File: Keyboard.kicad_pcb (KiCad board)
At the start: 2 copper layers, 50.8 x 59.5 mm, 36 parts, among them SW1 SW_Push, SW2 SW_Push, SW3 SW_Push, U1 ATmega32U2-AU, Y1 Crystal_GND24_Small

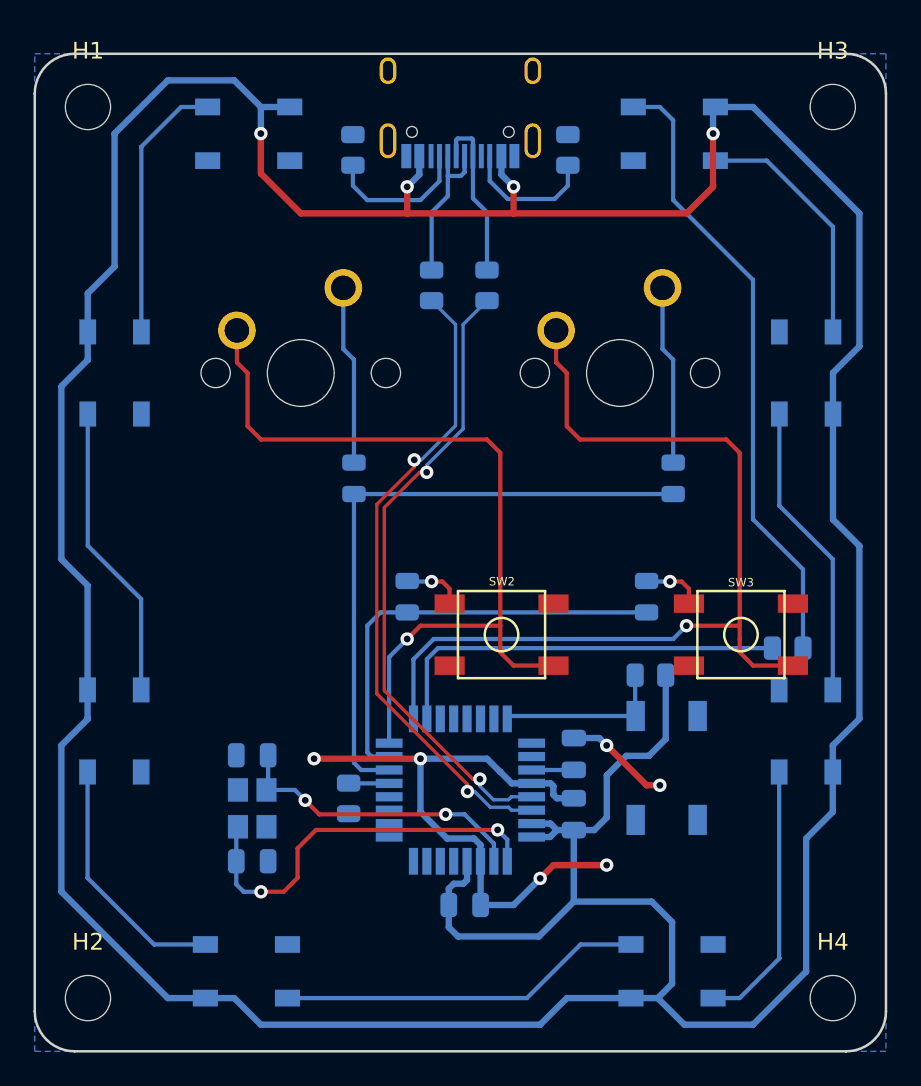
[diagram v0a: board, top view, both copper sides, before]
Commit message: Update Keyboard.kicad_pcb
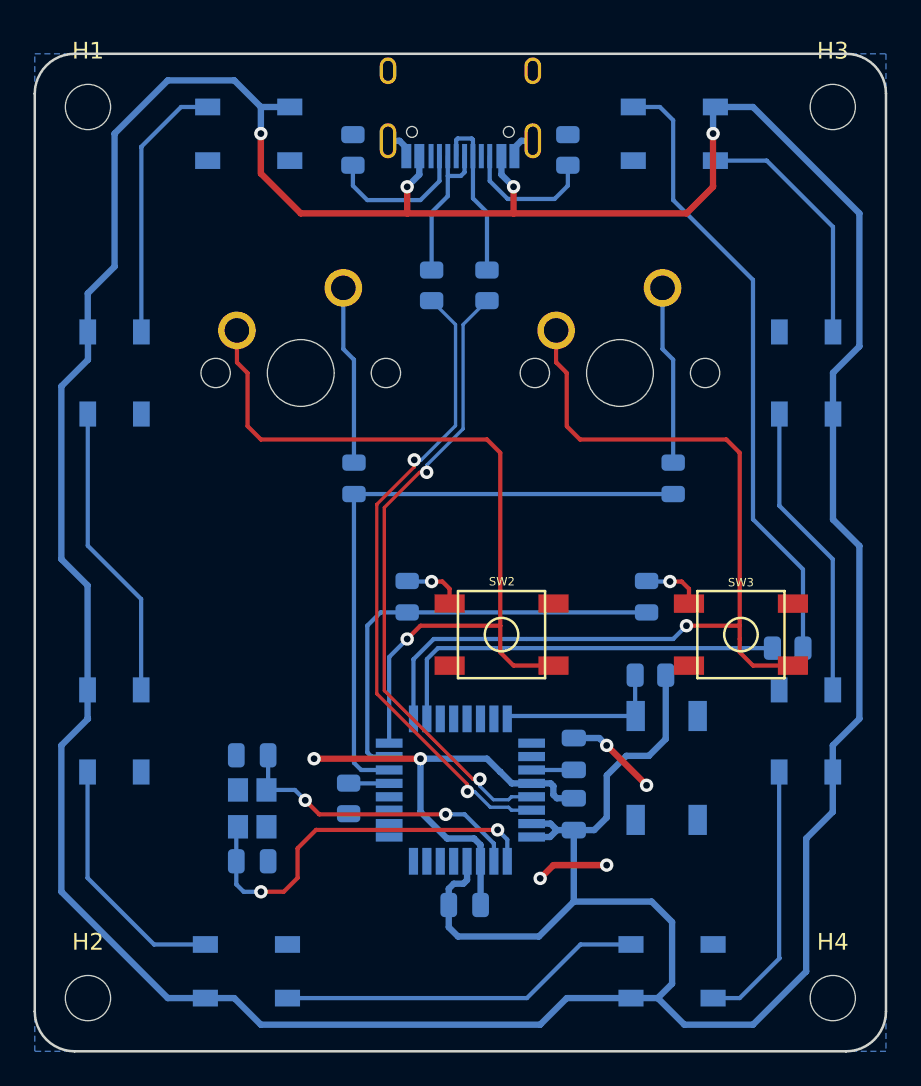
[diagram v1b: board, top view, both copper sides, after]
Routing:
- net GND: track 42.8 -> 41.3 mm
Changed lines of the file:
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@@
     (thickness 1.6)
     (drawings 8)
-    (tracks 302)
+    (tracks 306)
     (zones 0)
     (modules 36)
@@
   (segment (start 98.77925 78.9355) (end 99.21875 79.375) (width 0.381) (layer B.Cu) (net 2))
   (segment (start 97.2566 78.9355) (end 98.77925 78.9355) (width 0.381) (layer B.Cu) (net 2))
-  (via (at 102.39375 81.75625) (size 0.8) (drill 0.4) (layers F.Cu B.Cu) (net 2))
-  (segment (start 101.6 81.75625) (end 102.39375 81.75625) (width 0.381) (layer F.Cu) (net 2))
-  (segment (start 99.21875 79.375) (end 101.6 81.75625) (width 0.381) (layer F.Cu) (net 2))
   (via (at 95.25 87.3125) (size 0.8) (drill 0.4) (layers F.Cu B.Cu) (net 2))
-  (segment (start 93.6625 88.9) (end 95.25 87.3125) (width 0.381) (layer B.Cu) (net 2))
-  (segment (start 91.694 88.9) (end 93.6625 88.9) (width 0.381) (layer B.Cu) (net 2))
   (via (at 99.21875 86.51875) (size 0.8) (drill 0.4) (layers F.Cu B.Cu) (net 2))
   (segment (start 96.04375 86.51875) (end 99.21875 86.51875) (width 0.381) (layer F.Cu) (net 2))
@@
   (segment (start 92.075 80.16875) (end 88.10625 80.16875) (width 0.381) (layer B.Cu) (net 2))
   (segment (start 92.8605 80.95425) (end 92.075 80.16875) (width 0.381) (layer B.Cu) (net 2))
+  (via (at 101.6 81.75625) (size 0.8) (drill 0.4) (layers F.Cu B.Cu) (net 2))
+  (segment (start 99.21875 79.375) (end 101.6 81.75625) (width 0.381) (layer F.Cu) (net 2))
+  (segment (start 86.1675 43.2925) (end 86.1675 43.305) (width 0.381) (layer F.Cu) (net 2))
+  (segment (start 86.1675 43.2925) (end 86.8535 43.2925) (width 0.381) (layer B.Cu) (net 2))
+  (segment (start 87.2625 43.7015) (end 87.2625 44.2075) (width 0.381) (layer B.Cu) (net 2))
+  (segment (start 86.8535 43.2925) (end 87.2625 43.7015) (width 0.381) (layer B.Cu) (net 2))
+  (segment (start 94.8075 43.2925) (end 94.1215 43.2925) (width 0.381) (layer B.Cu) (net 2))
+  (segment (start 93.7125 43.7015) (end 93.7125 44.2075) (width 0.381) (layer B.Cu) (net 2))
+  (segment (start 94.1215 43.2925) (end 93.7125 43.7015) (width 0.381) (layer B.Cu) (net 2))
   (segment (start 77.1144 84.33435) (end 77.216 84.23275) (width 0.254) (layer B.Cu) (net 3))
   (segment (start 77.1144 86.29015) (end 77.1144 84.33435) (width 0.254) (layer B.Cu) (net 3))
@@
   (segment (start 68.25 52.4) (end 69.85 50.8) (width 0.381) (layer B.Cu) (net 5))
   (segment (start 68.25 54.7) (end 68.25 52.4) (width 0.381) (layer B.Cu) (net 5))
-  (segment (start 68.2625 56.35625) (end 68.25 56.34375) (width 0.381) (layer B.Cu) (net 5))
-  (segment (start 66.675 57.94375) (end 68.2625 56.35625) (width 0.381) (layer B.Cu) (net 5))
-  (segment (start 66.675 68.2625) (end 66.675 57.94375) (width 0.381) (layer B.Cu) (net 5))
-  (segment (start 68.25 56.34375) (end 68.25 54.7) (width 0.381) (layer B.Cu) (net 5))
-  (segment (start 68.2375 69.825) (end 66.675 68.2625) (width 0.381) (layer B.Cu) (net 5))
-  (segment (start 68.2375 76.0625) (end 68.2375 69.825) (width 0.381) (layer B.Cu) (net 5))
   (segment (start 68.2375 77.7625) (end 68.2375 76.0625) (width 0.381) (layer B.Cu) (net 5))
   (segment (start 68.2625 77.7875) (end 68.2375 77.7625) (width 0.381) (layer B.Cu) (net 5))
@@
   (segment (start 105.56875 41.4125) (end 105.70625 41.275) (width 0.381) (layer B.Cu) (net 5))
   (segment (start 105.56875 42.8625) (end 105.56875 41.4125) (width 0.381) (layer B.Cu) (net 5))
+  (segment (start 68.2375 69.825) (end 66.675 68.2625) (width 0.381) (layer B.Cu) (net 5))
+  (segment (start 68.2375 76.0625) (end 68.2375 69.825) (width 0.381) (layer B.Cu) (net 5))
+  (segment (start 66.675 68.2625) (end 66.675 57.94375) (width 0.381) (layer B.Cu) (net 5))
+  (segment (start 66.675 57.94375) (end 68.2625 56.35625) (width 0.381) (layer B.Cu) (net 5))
+  (segment (start 68.2625 54.7125) (end 68.25 54.7) (width 0.381) (layer B.Cu) (net 5))
+  (segment (start 68.2625 56.35625) (end 68.2625 54.7125) (width 0.381) (layer B.Cu) (net 5))
   (segment (start 83.5025 52.07) (end 83.5025 55.72125) (width 0.254) (layer B.Cu) (net 6))
   (segment (start 83.5025 55.72125) (end 84.1375 56.35625) (width 0.254) (layer B.Cu) (net 6))
